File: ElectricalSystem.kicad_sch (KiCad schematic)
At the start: 2 parts, among them SW3 Supp_Enable

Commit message: more stuff idk
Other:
- note added: "Array"
- note added: "HV Power Distribution"
- note added: "Main Battery Pack"
- note added: "Telemetry"
- note added: "add MPPTs, interface, blackbody A/C (temp/irradiance sensors)"
- note added: "add dynamics, environment, TPMS transceiver, broker?"
- note added: "replace with VCU and new architecture"
- note removed: "Battery"
- moved on the sheet: SW3

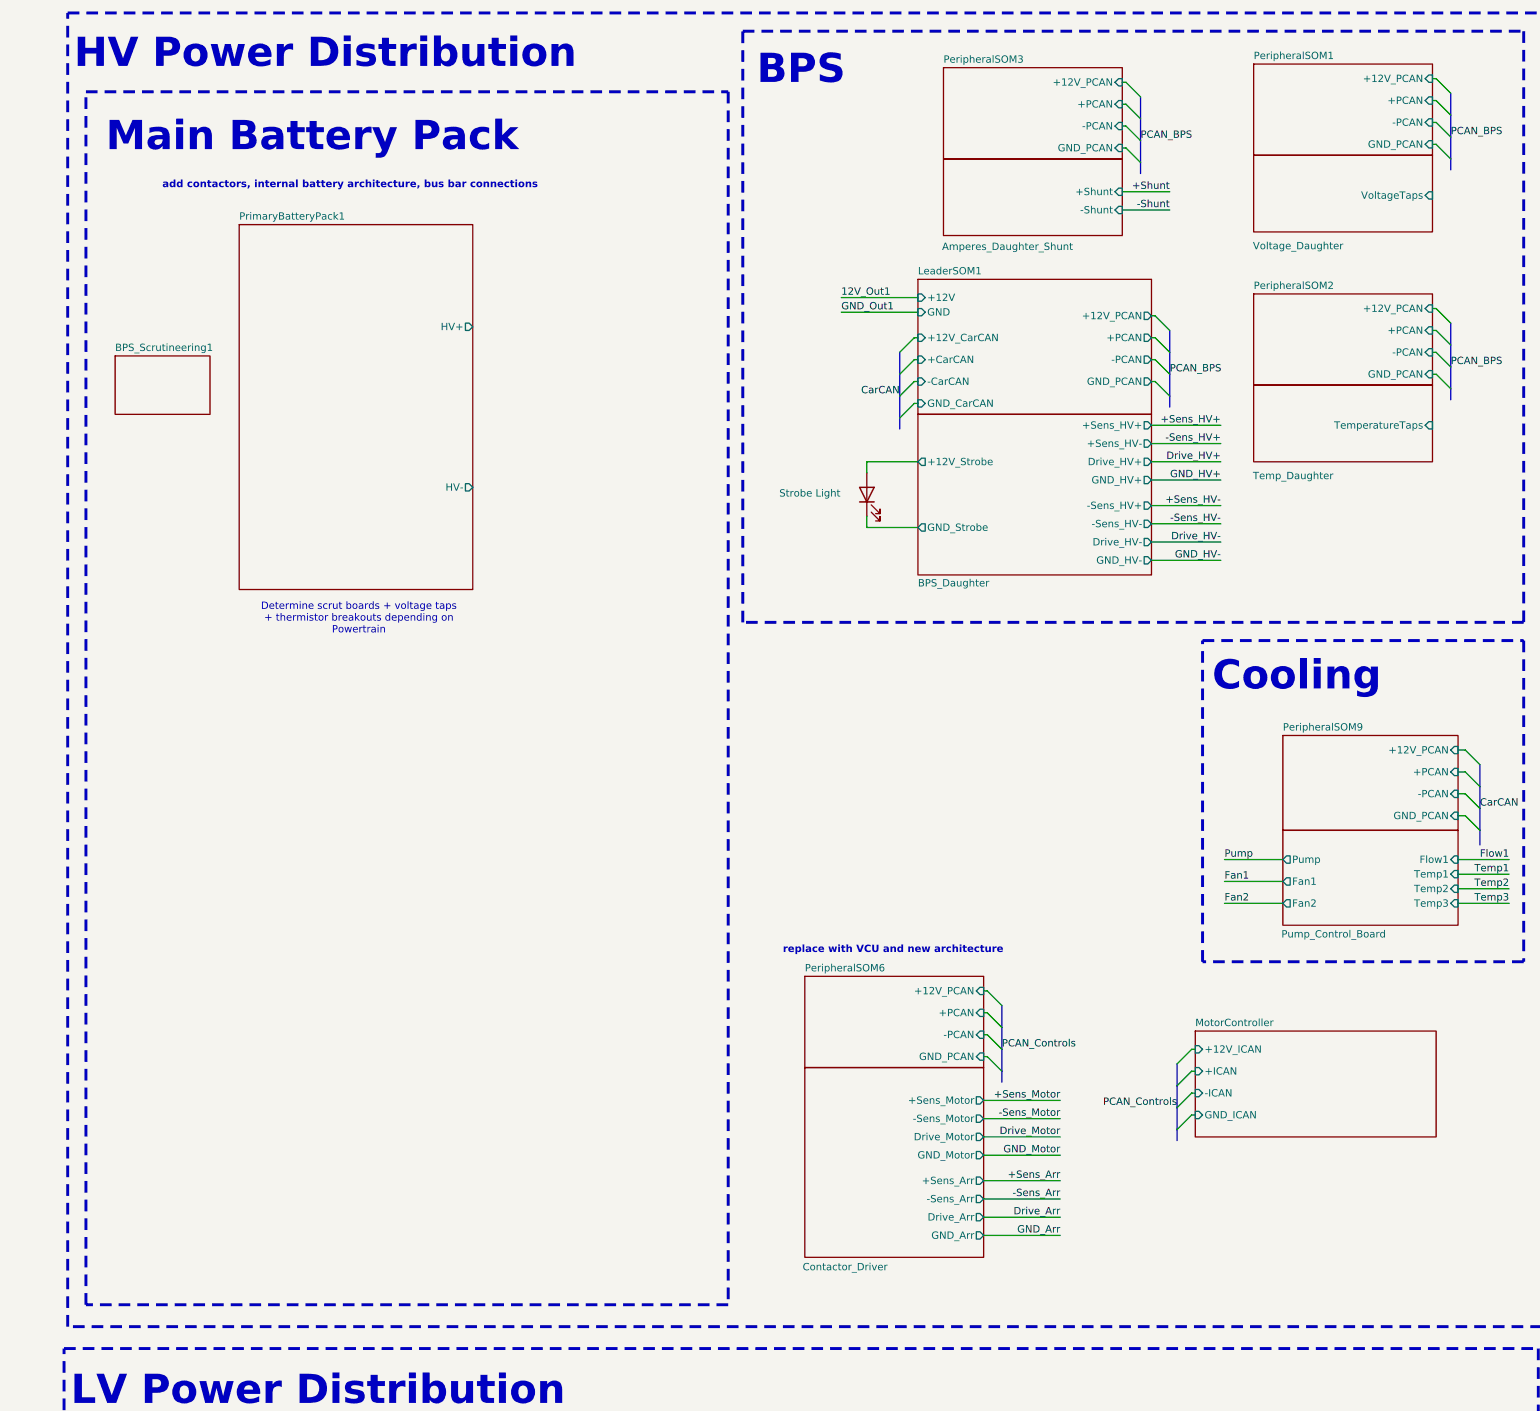
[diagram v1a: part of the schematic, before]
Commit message: heheheheh
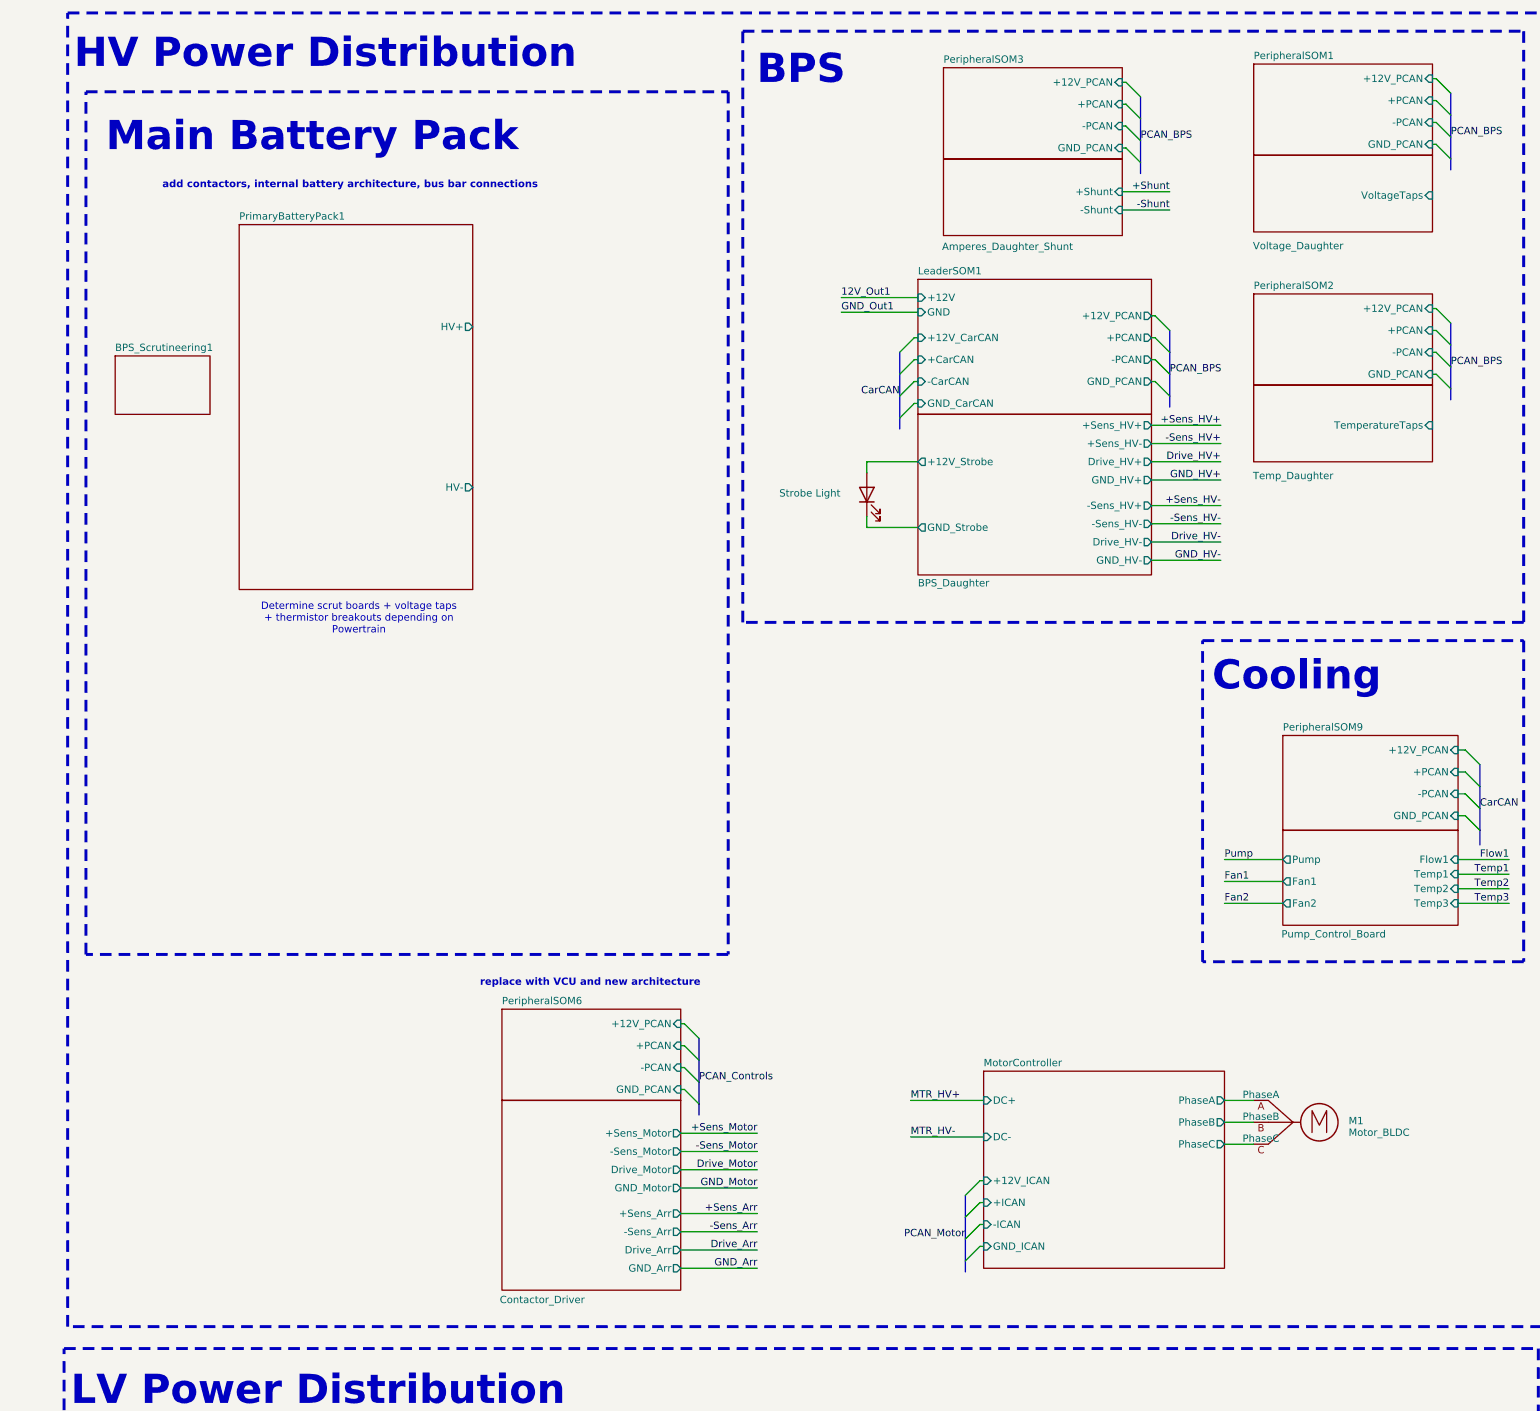
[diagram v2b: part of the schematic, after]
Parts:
- added M1: Motor_BLDC, symbol Motor:Motor_DC
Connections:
- new net MotorController/PhaseA: M1.A (PhaseA)
- new net MotorController/PhaseB: M1.B (PhaseB)
- new net MotorController/PhaseC: M1.C (PhaseC)
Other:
- sheet MotorController ports: added DC+, DC-, PhaseA, PhaseB, PhaseC; removed none
